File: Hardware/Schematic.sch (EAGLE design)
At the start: 103 parts, among them IC1 BD5229G-TR, IC4 XC6220A331MR-G, J1 FH34SRJ-24S-0.5SH_99_, J2 SAMACSYS_PARTS_USB4110-GF-A, J3 QWIIC_RIGHT_ANGLE, J4 112A-TAAR-R03_ATTEND, Q1 20V/4.2A/52mΩ/1.4W, Q2 20V/4.2A/52mΩ/1.4W, Q3 SI1308EDL-T1-GE3, U1 W25Q512JVEIQ, U2 ESP32-C6-WROOM-1-N8, U3 DS3231SN#, U4 MAX17048G+T10

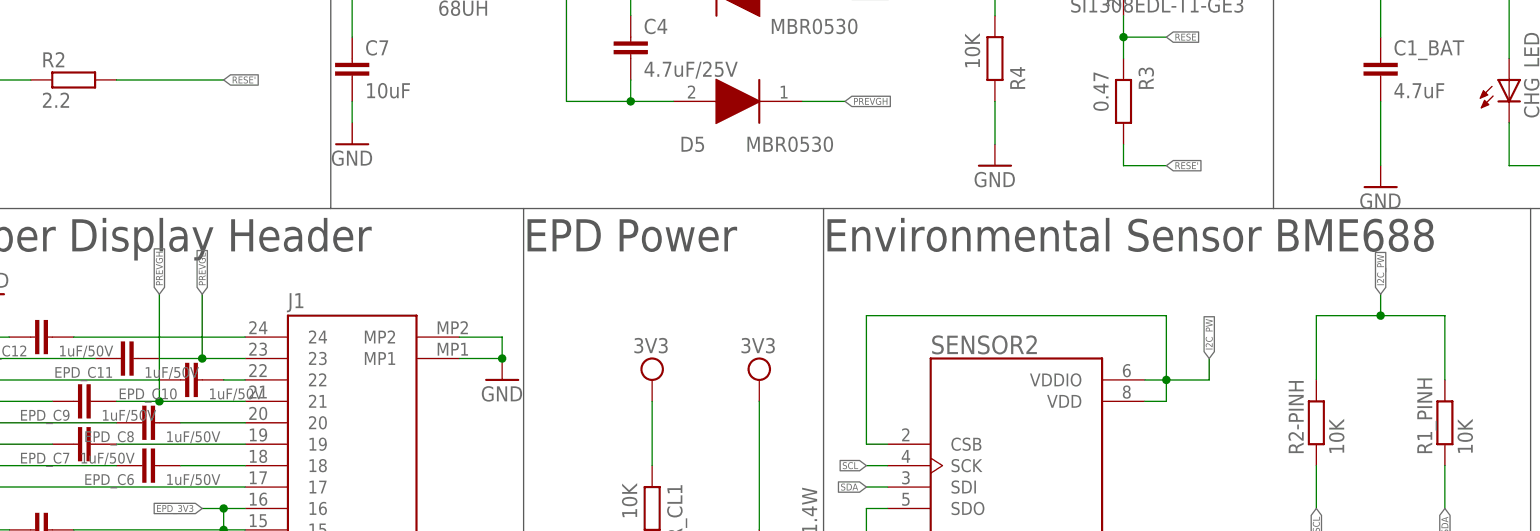
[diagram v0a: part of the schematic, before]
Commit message: Fixed issues
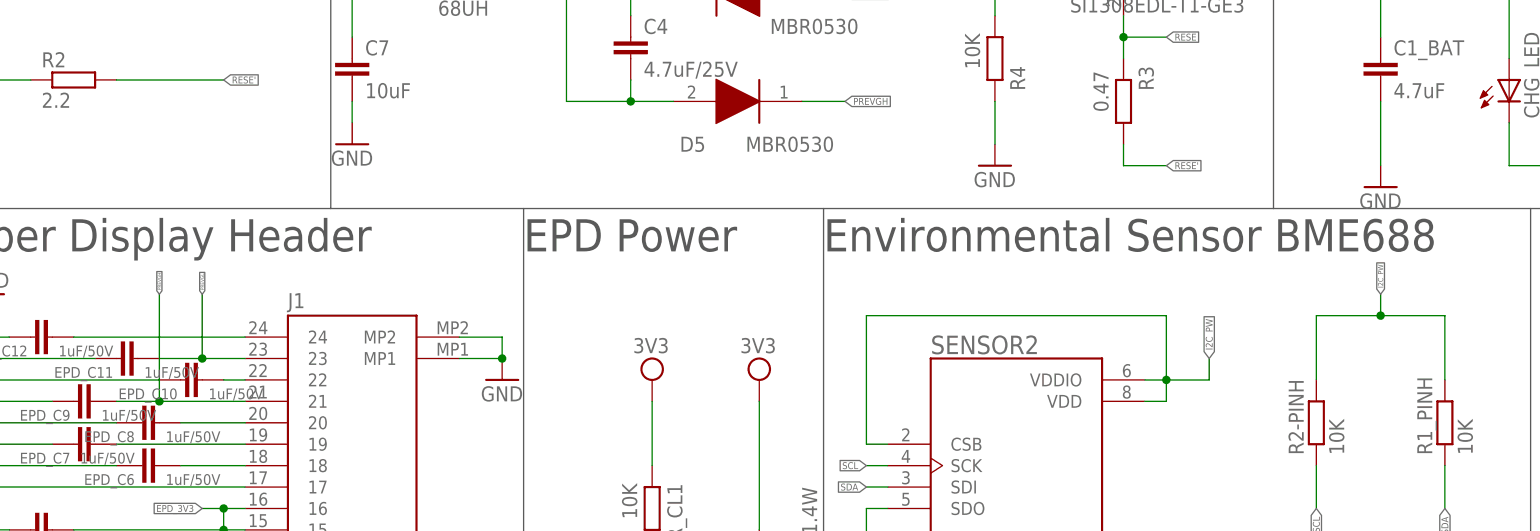
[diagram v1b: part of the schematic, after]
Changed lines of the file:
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@@
 <part name="GND13" library="DeskAssistant v19 v1" library_urn="urn:adsk.wipprod:fs.file:vf.xl3ZwHFcSImjuActhDYHeQ" deviceset="GND" device=""/>
 <part name="GND14" library="DeskAssistant v19 v1" library_urn="urn:adsk.wipprod:fs.file:vf.xl3ZwHFcSImjuActhDYHeQ" deviceset="GND" device=""/>
-<part uuid="2882400001" name="L1" library="DeskAssistant v19 v1" library_urn="urn:adsk.wipprod:fs.file:vf.xl3ZwHFcSImjuActhDYHeQ" deviceset="744043680" device="IND_4828-WE-TPC_WRE">
+<part uuid="2882400001" name="L1" library="DeskAssistant v19 v1" library_urn="urn:adsk.wipprod:fs.file:vf.xl3ZwHFcSImjuActhDYHeQ" deviceset="744043680" device="IND_4828-WE-TPC_WRE" package3d_urn="urn:adsk.eagle:package:47640298/1" override_locally_modified="yes" value="744043680IND_4828-WE-TPC_WRE">
 <attribute name="68UH" value="68UH"/>
 </part>
@@
 <pinref part="C7" gate="G$1" pin="1"/>
 <wire x1="45.72" y1="12.7" x2="45.72" y2="17.78" width="0.1524" layer="91"/>
-<pinref part="L1" gate="A" pin="2"/>
 <wire x1="45.72" y1="17.78" x2="45.72" y2="20.32" width="0.1524" layer="91"/>
 <wire x1="50.8" y1="17.78" x2="45.72" y2="17.78" width="0.1524" layer="91"/>
 <junction x="45.72" y="17.78"/>
 <label x="45.72" y="20.32" size="0.8128" layer="95" rot="R90" xref="yes"/>
+<pinref part="L1" gate="A" pin="2"/>
 </segment>
 <segment>
@@
 <net name="SRC" class="0">
 <segment>
-<pinref part="L1" gate="A" pin="1"/>
 <wire x1="66.04" y1="17.78" x2="68.58" y2="17.78" width="0.1524" layer="91"/>
 <wire x1="68.58" y1="22.86" x2="68.58" y2="17.78" width="0.1524" layer="91"/>
@@
 <junction x="78.74" y="5.08"/>
 <label x="68.58" y="22.86" size="0.8128" layer="95" rot="R90" xref="yes"/>
+<pinref part="L1" gate="A" pin="1"/>
 </segment>
 <segment>
@@
 <junction x="27.94" y="-25.4"/>
 <wire x1="27.94" y1="-25.4" x2="27.94" y2="-17.78" width="0.1524" layer="91"/>
-<label x="27.94" y="-17.78" size="0.8128" layer="95" rot="R90" xref="yes"/>
+<label x="27.94" y="-17.78" size="0.4064" layer="95" rot="R90" xref="yes"/>
 </segment>
 </net>
@@
 <junction x="22.86" y="-30.48"/>
 <wire x1="22.86" y1="-30.48" x2="22.86" y2="-17.78" width="0.1524" layer="91"/>
-<label x="22.86" y="-17.78" size="0.8128" layer="95" rot="R90" xref="yes"/>
+<label x="22.86" y="-17.78" size="0.4064" layer="95" rot="R90" xref="yes"/>
 </segment>
 </net>
@@
 <junction x="167.64" y="-20.32"/>
 <wire x1="167.64" y1="-20.32" x2="167.64" y2="-17.78" width="0.1524" layer="91"/>
-<label x="167.64" y="-17.78" size="0.8128" layer="95" rot="R90" xref="yes"/>
-</segment>
-<segment>
+<label x="167.64" y="-17.78" size="0.6096" layer="95" rot="R90" xref="yes"/>
+</segment>
+<segment>
